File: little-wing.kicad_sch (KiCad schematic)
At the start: 71 parts, among them IC1 AP7335-WG-7, J1 Conn_01x08, SW1 Power, SW2 Reset, U1 Nice_Nano_V2, U2 PMW3610

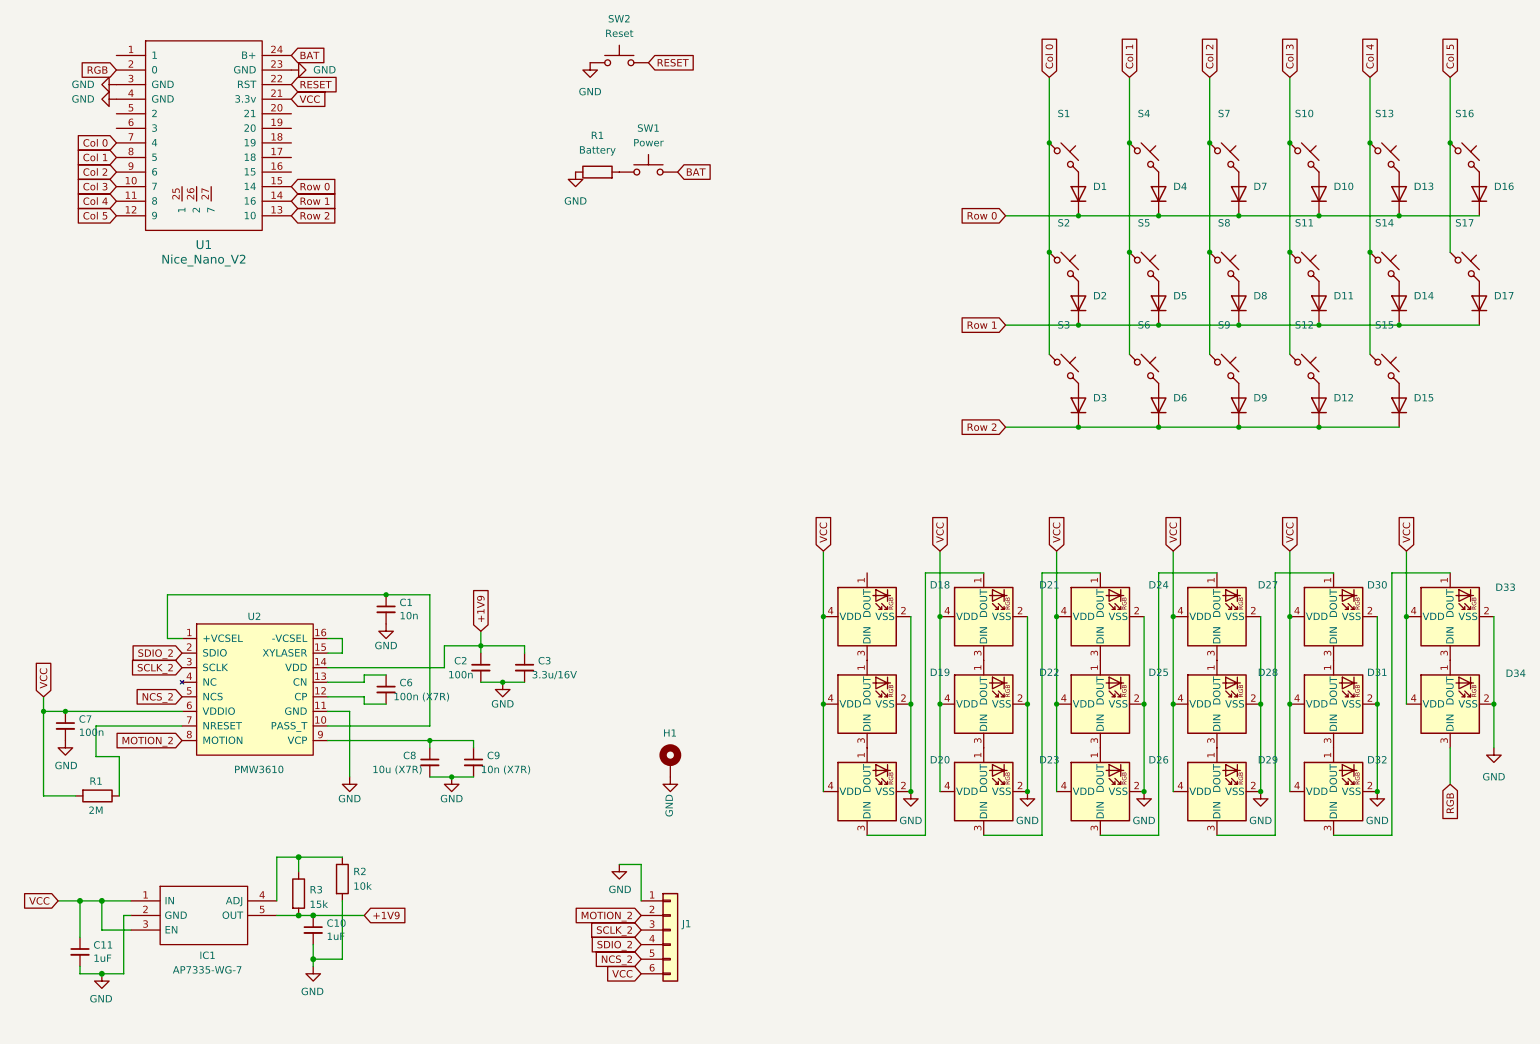
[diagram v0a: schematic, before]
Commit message: Initial PCB layout
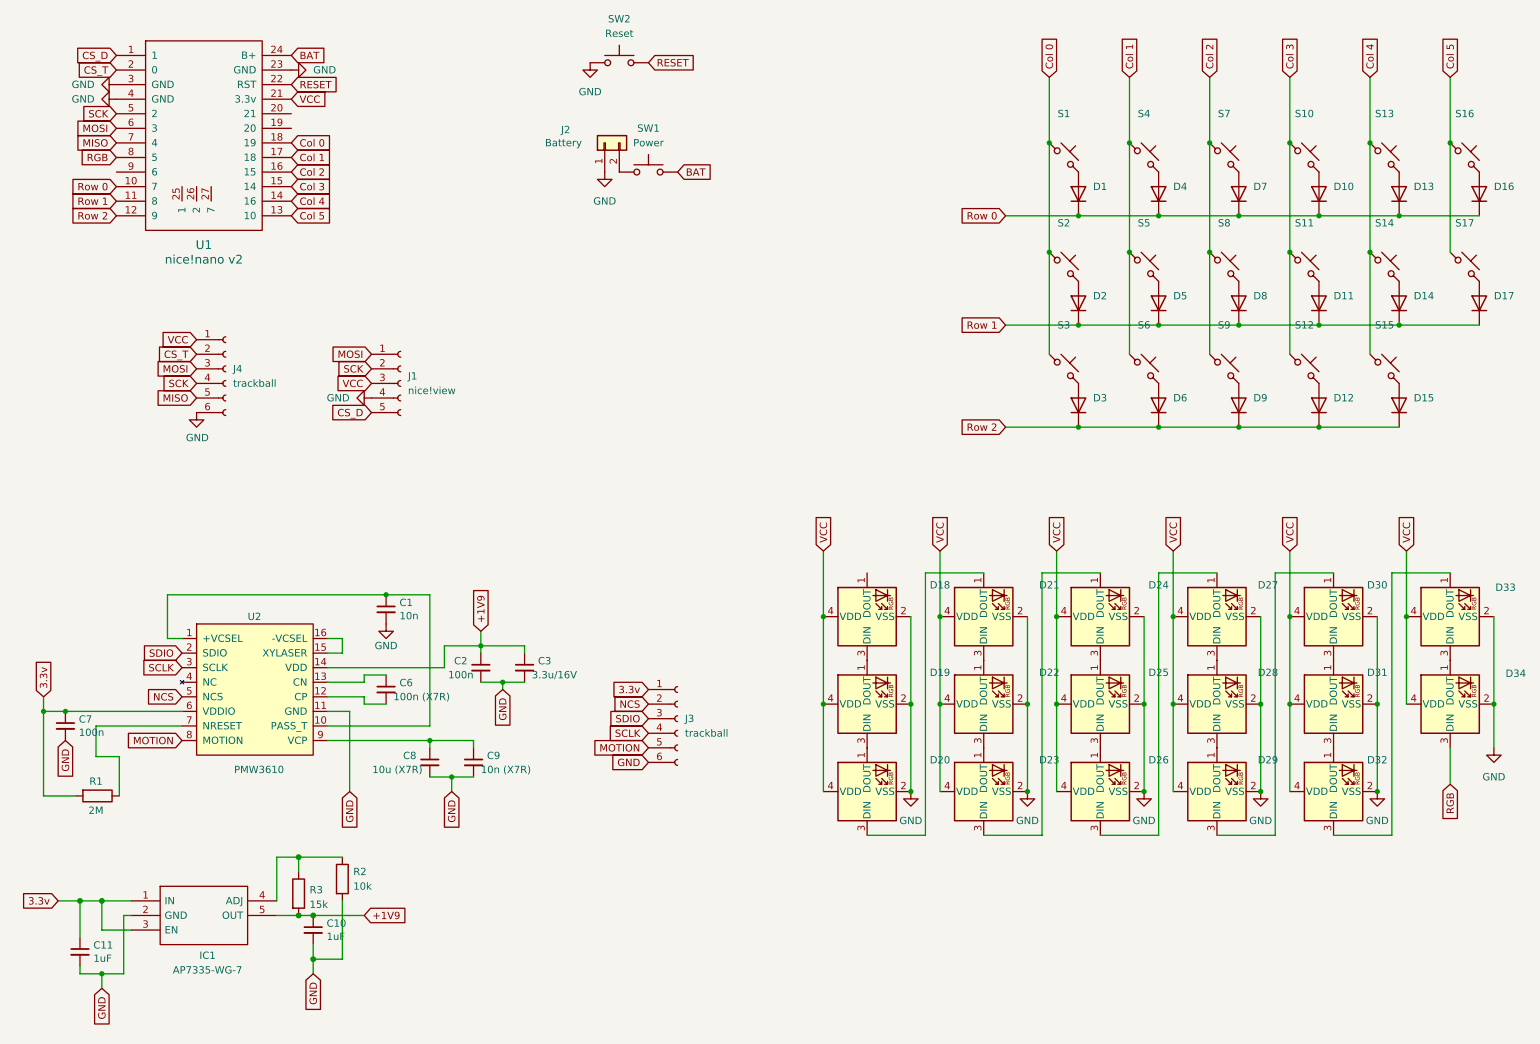
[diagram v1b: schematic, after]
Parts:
- removed H1: NA_M4, local-libraries:MountingHole_3mm_Pad_Via, symbol Mechanical:MountingHole_Pad
- removed J1: Conn_01x08, Connector_PinHeader_2.54mm:PinHeader_1x06_P2.54mm_Vertical, symbol Connector_Generic:Conn_01x06
- removed R1: Battery, symbol ScottoKeebs:Placeholder_Resistor
- added J1: nice!view, Connector_Wire:SolderWire-0.1sqmm_1x05_P3.6mm_D0.4mm_OD1mm, symbol Connector:Conn_01x05_Socket
- added J2: Battery, Connector_JST:JST_PH_S2B-PH-K_1x02_P2.00mm_Horizontal, symbol Connector_Generic:Conn_01x02
- added J3, J4: trackball, Connector_Wire:SolderWire-0.1sqmm_1x06_P3.6mm_D0.4mm_OD1mm, symbol Connector:Conn_01x06_Socket
- C10, C11: footprint lib:C_0603_1608Metric -> Capacitor_SMD:C_0603_1608Metric
- D1, D10, D11, D12, D13, D14, D15, D16, D17, D2, D3, D4, D5, D6, D7, D8, D9: footprint (none) -> Diode_SMD:D_0603_1608Metric
- R2, R3: footprint lib:R_0603_1608Metric -> Resistor_SMD:R_0603_1608Metric
- S1, S10, S11, S12, S13, S14, S15, S16, S17, S2, S3, S4, S5, S6, S7, S8, S9: footprint (none) -> keyswitches:Kailh_socket_PG1350_reversible
- SW1: footprint (none) -> switch:switch-MSK-12C02-smd
- SW2: footprint (none) -> ScottoKeebs_Components:Button_MJTP1243
- U1: value Nice_Nano_V2 -> nice!nano v2; footprint ScottoKeebs_MCU:Nice_Nano_V2 -> keyboard_reversible:ProMicro
- U2: footprint mylib:PMW3610 -> sensor:PMW3610
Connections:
- net Col 0: now also U1.18 (19); no longer U1.7 (4)
- net Col 1: now also U1.17 (18); no longer U1.8 (5)
- net Col 2: now also U1.16 (15); no longer U1.9 (6)
- net Col 3: now also U1.15 (14); no longer U1.10 (7)
- net Col 4: now also U1.14 (16); no longer U1.11 (8)
- net Col 5: now also U1.13 (10); no longer U1.12 (9)
- net GND: now also J1.4 (Pin_4), J2.1 (Pin_1), J3.6 (Pin_6), J4.6 (Pin_6)
- net RGB: now also U1.8 (5); no longer U1.2 (0)
- net Row 0: now also U1.10 (7); no longer U1.15 (14)
- net Row 1: now also U1.11 (8); no longer U1.14 (16)
- net Row 2: now also U1.12 (9); no longer U1.13 (10)
- net VCC: now also J1.3 (Pin_3), J4.1 (Pin_1); no longer C11.1, C7.1, IC1.1 (IN), IC1.3 (EN), R1.2, U2.6 (VDDIO)
- net CS_D: now reaches U1.1
- net CS_D: now also J1.5 (Pin_5)
- net SCK: now reaches U1.5 (2)
- net SCK: now also J1.2 (Pin_2), J4.4 (Pin_4)
- net MOSI: now reaches U1.6 (3)
- net MOSI: now also J1.1 (Pin_1), J4.3 (Pin_3)
- net at SW1.1: now also J2.2 (Pin_2)
- net MOTION_2 renamed MOTION
- net MOTION: now also J3.5 (Pin_5)
- net NCS_2 renamed NCS
- net NCS: now also J3.2 (Pin_2)
- net SCLK_2 renamed SCLK
- net SCLK: now also J3.4 (Pin_4)
- net SDIO_2 renamed SDIO
- net SDIO: now also J3.3 (Pin_3)
- new net 3.3v: C11.1, C7.1, IC1.1 (IN), IC1.3 (EN), J3.1 (Pin_1), R1.2, U2.6 (VDDIO)
- new net CS_T: J4.2 (Pin_2), U1.2 (0)
- new net MISO: J4.5 (Pin_5), U1.7 (4)
